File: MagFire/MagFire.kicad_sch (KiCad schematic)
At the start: 5 parts, among them J1 Conn_01x01, SW1 SW_Push, SW2 SW_Push

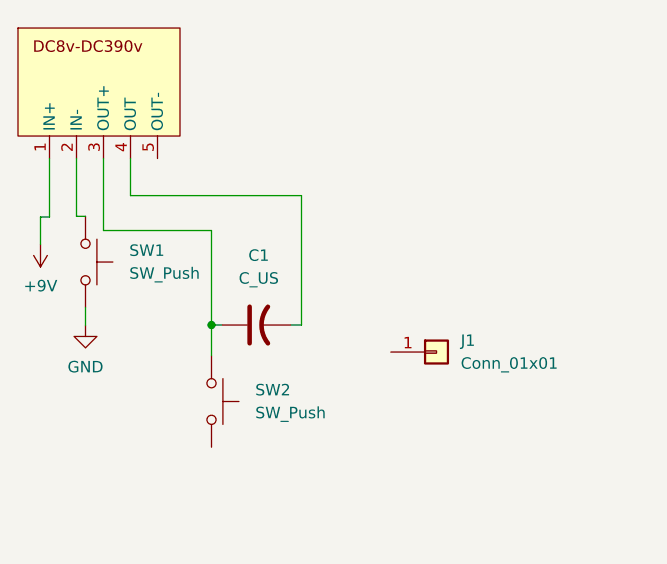
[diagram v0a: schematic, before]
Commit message: update model and pcb and journal
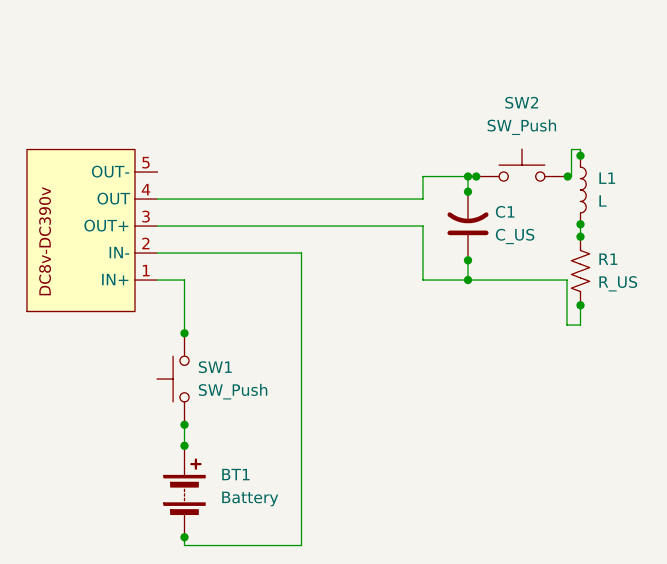
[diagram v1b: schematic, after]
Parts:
- removed J1: Conn_01x01, symbol Connector_Generic:Conn_01x01
- added BT1: Battery, Connector_Wire:SolderWire-0.75sqmm_1x02_P7mm_D1.25mm_OD3.5mm, symbol Device:Battery
- added L1: L, Connector_Wire:SolderWire-0.75sqmm_1x02_P7mm_D1.25mm_OD3.5mm, symbol Device:L
- added R1: R_US, Connector_Wire:SolderWire-0.75sqmm_1x02_P7mm_D1.25mm_OD3.5mm, symbol Device:R_US
- C1: footprint (none) -> Capacitor_THT:CP_Radial_D35.0mm_P10.00mm_SnapIn
- SW1, SW2: footprint (none) -> Connector_Wire:SolderWire-0.75sqmm_1x02_P7mm_D1.25mm_OD3.5mm
- U1: footprint (none) -> KS_Maker:DC-DC390v_transformer_3
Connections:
- net GND is gone; now on an unnamed net: SW1.2
- net at C1.1, U1.3 (OUT+): now also R1.2; no longer SW2.1
- net at C1.2, U1.4 (OUT): now also SW2.1
- net at U1.2 (IN-): now also BT1.2 (-); no longer SW1.1
- net at SW2.2: now also L1.1
- net +9V: no longer names the net of U1.1 (IN+)
- new net: L1.2, R1.1
- new net: BT1.1 (+), SW1.1

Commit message: update everything
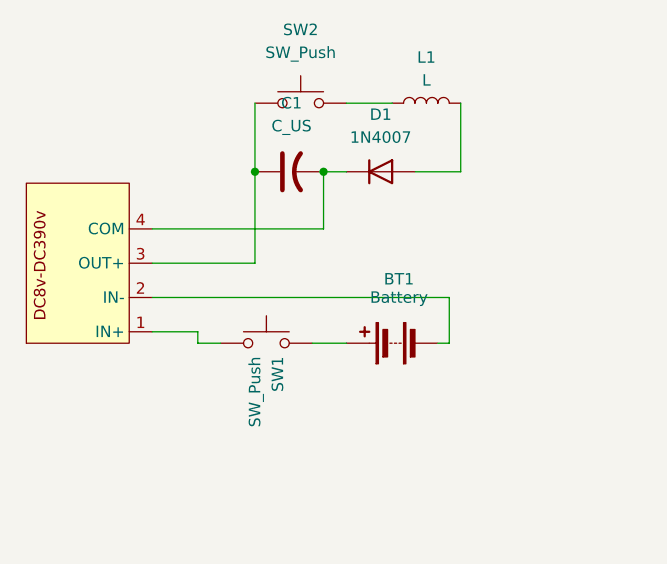
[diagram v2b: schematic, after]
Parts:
- removed R1: R_US, Connector_Wire:SolderWire-0.75sqmm_1x02_P7mm_D1.25mm_OD3.5mm, symbol Device:R_US
- added D1: 1N4007, Diode_THT:D_DO-41_SOD81_P10.16mm_Horizontal, symbol Diode:1N4007
- U1: footprint KS_Maker:DC-DC390v_transformer_3 -> (none)
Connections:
- net at C1.2, U1.4 (COM): now also D1.1 (K); no longer SW2.1
- net at L1.2: now also D1.2 (A)
- net at C1.1, U1.3 (OUT+): now also SW2.1
- net at U1.1 (IN+): now also SW1.1; no longer SW1.2
- net at BT1.1 (+): now also SW1.2; no longer SW1.1
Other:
- moved on the sheet: BT1, C1, L1, SW1, SW2
